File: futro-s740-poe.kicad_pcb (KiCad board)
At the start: 4 copper layers, 79.5 x 30 mm, 9 parts, among them J1 Conn_02x08, J2 Conn_02x08, U1 SM51589PEL, U2 AG5412

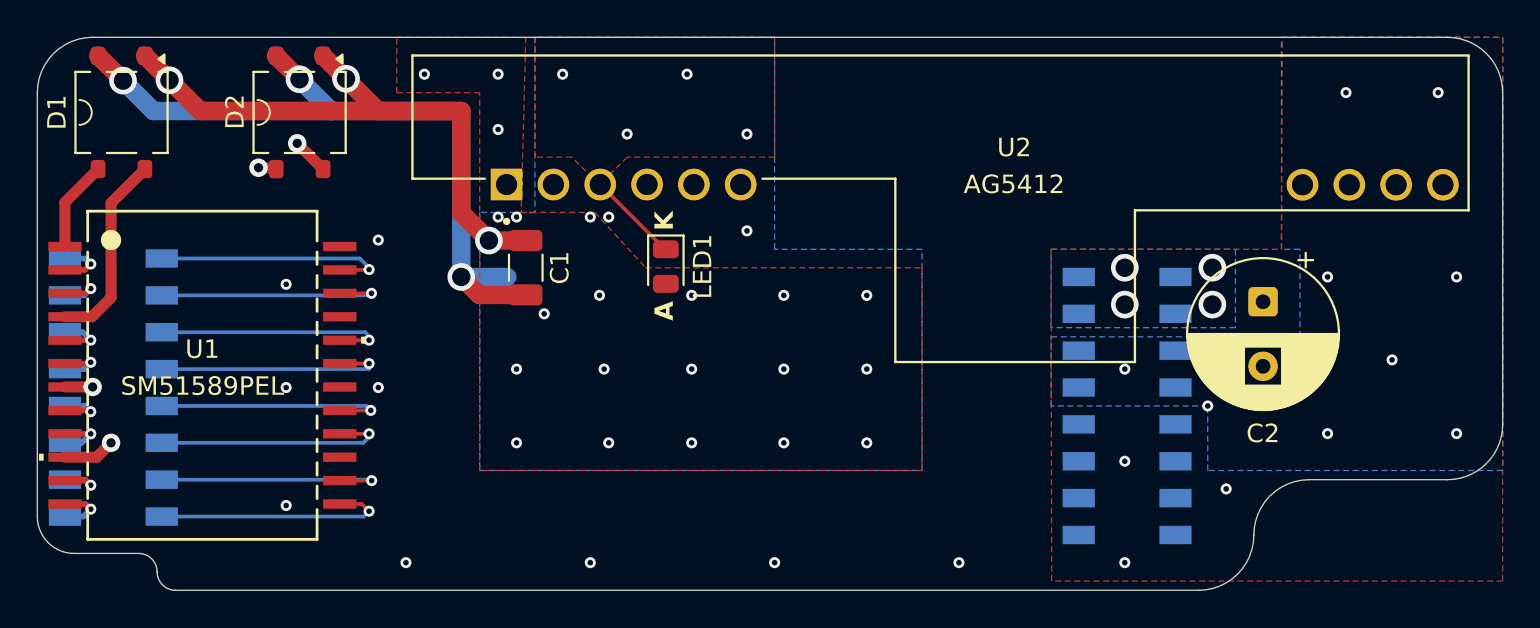
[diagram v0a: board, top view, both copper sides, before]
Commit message: tweak
Signed-off-by: Takuto Nagami <logica0419@gmail.com>
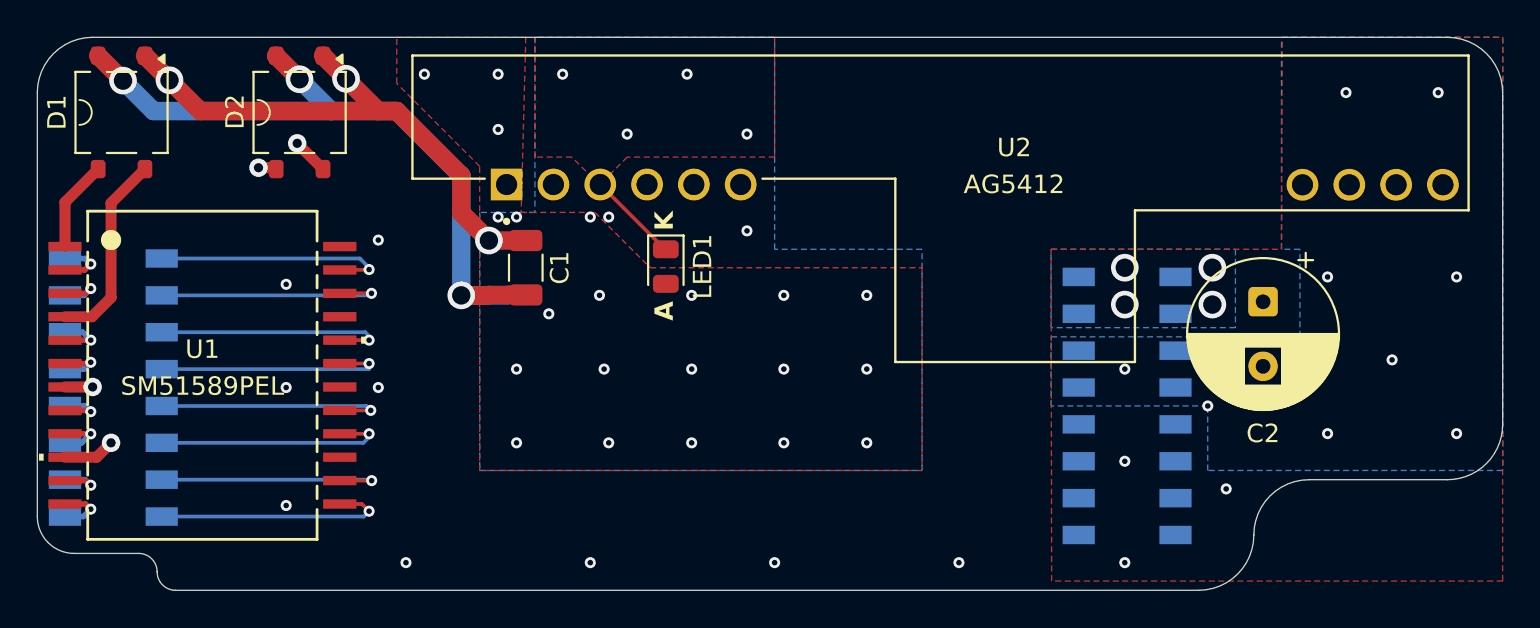
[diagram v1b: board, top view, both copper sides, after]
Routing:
- net Net-(D1-+): track 63.4 -> 55.8 mm
- net Net-(D1--): track 74.6 -> 72.1 mm
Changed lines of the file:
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@@
+	)
+	(segment
+		(start 28.84 22)
+		(end 39.5 22)
+		(width 1)
+		(layer "F.Cu")
+		(net "Net-(D1-+)")
+	)
+	(segment
+		(start 38.5 22)
+		(end 35.5 19)
+		(width 1)
+		(layer "F.Cu")
+		(net "Net-(D1-+)")
+	)
+	(segment
+		(start 39.5 22)
+		(end 43 25.5)
+		(width 1)
+		(layer "F.Cu")
+		(net "Net-(D1-+)")
 	)
 	(segment
@@
 	)
 	(segment
-		(start 43 22)
-		(end 43 27.525)
+		(start 44.5 29.025)
+		(end 46.5 29.025)
 		(width 1)
 		(layer "F.Cu")
@@
 	)
 	(segment
-		(start 44.5 29.025)
-		(end 46.5 29.025)
-		(width 1)
-		(layer "F.Cu")
-		(net "Net-(D1-+)")
-	)
-	(segment
-		(start 28.84 22)
-		(end 43 22)
-		(width 1)
-		(layer "F.Cu")
-		(net "Net-(D1-+)")
-	)
-	(segment
-		(start 35.5 19)
+		(start 43 25.5)
+		(end 43 27.525)
+		(width 1)
+		(layer "F.Cu")
+		(net "Net-(D1-+)")
+	)
+	(segment
+		(start 39.5 22)
 		(end 38.5 22)
-		(width 1)
-		(layer "F.Cu")
-		(net "Net-(D1-+)")
-	)
-	(segment
-		(start 38.5 22)
-		(end 43 22)
 		(width 1)
 		(layer "F.Cu")
@@
 	)
 	(segment
-		(start 43 22)
+		(start 43 25.5)
 		(end 43 27.525)
+		(width 1)
+		(layer "In1.Cu")
+		(net "Net-(D1-+)")
+	)
+	(segment
+		(start 39.5 22)
+		(end 43 25.5)
 		(width 1)
 		(layer "In1.Cu")
@@
 	)
 	(segment
+		(start 38.5 22)
+		(end 39.5 22)
+		(width 1)
+		(layer "In1.Cu")
+		(net "Net-(D1-+)")
+	)
+	(segment
 		(start 27.17 20.33)
 		(end 28.84 22)
@@
 	)
 	(segment
-		(start 38.5 22)
-		(end 43 22)
-		(width 1)
-		(layer "In1.Cu")
-		(net "Net-(D1-+)")
+		(start 44.475 31.975)
+		(end 46.5 31.975)
+		(width 1)
+		(layer "F.Cu")
+		(net "Net-(D1--)")
 	)
 	(segment
@@
 	)
 	(segment
+		(start 44.45 32)
+		(end 44.475 31.975)
+		(width 1)
+		(layer "F.Cu")
+		(net "Net-(D1--)")
+	)
+	(segment
 		(start 34.225 20.275)
 		(end 32.96 19.01)
@@
 	)
 	(segment
-		(start 43.975 31.975)
-		(end 46.5 31.975)
+		(start 43 32)
+		(end 44.45 32)
 		(width 1)
 		(layer "F.Cu")
@@
 	)
 	(segment
-		(start 43 31)
-		(end 43.975 31.975)
-		(width 1)
-		(layer "F.Cu")
-		(net "Net-(D1--)")
-	)
-	(segment
 		(start 46.5 31.975)
 		(end 45.5 31.975)
@@
 	)
 	(via
-		(at 47.5 33)
+		(at 47.75 33)
 		(size 0.6)
 		(drill 0.3)
@@
 	)
 	(via
-		(at 43 31)
+		(at 43 32)
 		(size 1.5)
 		(drill 1)
@@
 	)
 	(segment
-		(start 26.3 22)
-		(end 43 22)
-		(width 1)
-		(layer "B.Cu")
-		(net "Net-(D1--)")
-	)
-	(segment
 		(start 34.225 20.275)
 		(end 35.95 22)
@@
 	)
 	(segment
+		(start 39.5 22)
+		(end 26.3 22)
+		(width 1)
+		(layer "B.Cu")
+		(net "Net-(D1--)")
+	)
+	(segment
+		(start 43 32)
+		(end 45.5 32)
+		(width 1)
+		(layer "B.Cu")
+		(net "Net-(D1--)")
+	)
+	(segment
+		(start 43 32)
+		(end 43 25.5)
+		(width 1)
+		(layer "B.Cu")
+		(net "Net-(D1--)")
+	)
+	(segment
+		(start 43 25.5)
+		(end 39.5 22)
+		(width 1)
+		(layer "B.Cu")
+		(net "Net-(D1--)")
+	)
+	(segment
+		(start 26.3 22)
+		(end 24.65 20.35)
+		(width 1)
+		(layer "B.Cu")
+		(net "Net-(D1--)")
+	)
+	(segment
+		(start 26.3 22)
+		(end 35.95 22)
+		(width 1)
+		(layer "In2.Cu")
+		(net "Net-(D1--)")
+	)
+	(segment
+		(start 34.225 20.275)
+		(end 35.95 22)
+		(width 1)
+		(layer "In2.Cu")
+		(net "Net-(D1--)")
+	)
+	(segment
+		(start 43 25.5)
+		(end 39.5 22)
+		(width 1)
+		(layer "In2.Cu")
+		(net "Net-(D1--)")
+	)
+	(segment
+		(start 39.5 22)
+		(end 35.95 22)
+		(width 1)
+		(layer "In2.Cu")
+		(net "Net-(D1--)")
+	)
+	(segment
+		(start 43 32)
+		(end 43 25.5)
+		(width 1)
+		(layer "In2.Cu")
+		(net "Net-(D1--)")
+	)
+	(segment
+		(start 43 32)
+		(end 45.5 32)
+		(width 1)
+		(layer "In2.Cu")
+		(net "Net-(D1--)")
+	)
+	(segment
 		(start 24.65 20.35)
 		(end 26.3 22)
-		(width 1)
-		(layer "B.Cu")
-		(net "Net-(D1--)")
-	)
-	(segment
-		(start 43 22)
-		(end 43 31)
-		(width 1)
-		(layer "B.Cu")
-		(net "Net-(D1--)")
-	)
-	(segment
-		(start 43 31)
-		(end 45.5 31)
-		(width 1)
-		(layer "B.Cu")
-		(net "Net-(D1--)")
-	)
-	(segment
-		(start 26.3 22)
-		(end 35.95 22)
-		(width 1)
-		(layer "In2.Cu")
-		(net "Net-(D1--)")
-	)
-	(segment
-		(start 43 22)
-		(end 43 31)
-		(width 1)
-		(layer "In2.Cu")
-		(net "Net-(D1--)")
-	)
-	(segment
-		(start 34.225 20.275)
-		(end 35.95 22)
-		(width 1)
-		(layer "In2.Cu")
-		(net "Net-(D1--)")
-	)
-	(segment
-		(start 35.95 22)
-		(end 43 22)
-		(width 1)
-		(layer "In2.Cu")
-		(net "Net-(D1--)")
-	)
-	(segment
-		(start 24.65 20.35)
-		(end 26.3 22)
-		(width 1)
-		(layer "In2.Cu")
-		(net "Net-(D1--)")
-	)
-	(segment
-		(start 43 31)
-		(end 45.5 31)
 		(width 1)
 		(layer "In2.Cu")
@@
 		(polygon
 			(pts
-				(xy 44 21) (xy 39.5 21) (xy 39.5 18) (xy 46.5 18) (xy 46.25 27.5) (xy 50.25 27.5) (xy 53 30.5) (xy 68 30.5)
-				(xy 68 41.5) (xy 44 41.5)
+				(xy 44 25) (xy 39.5 20.5) (xy 39.5 18) (xy 46.5 18) (xy 46.25 27.5) (xy 50.25 27.5) (xy 53.25 30.5)
+				(xy 68 30.5) (xy 68 41.5) (xy 44 41.5)
 			)
 		)
